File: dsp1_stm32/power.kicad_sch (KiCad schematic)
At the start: 41 parts, among them U10 TLV62568DBV, U9 TLV62568DBV

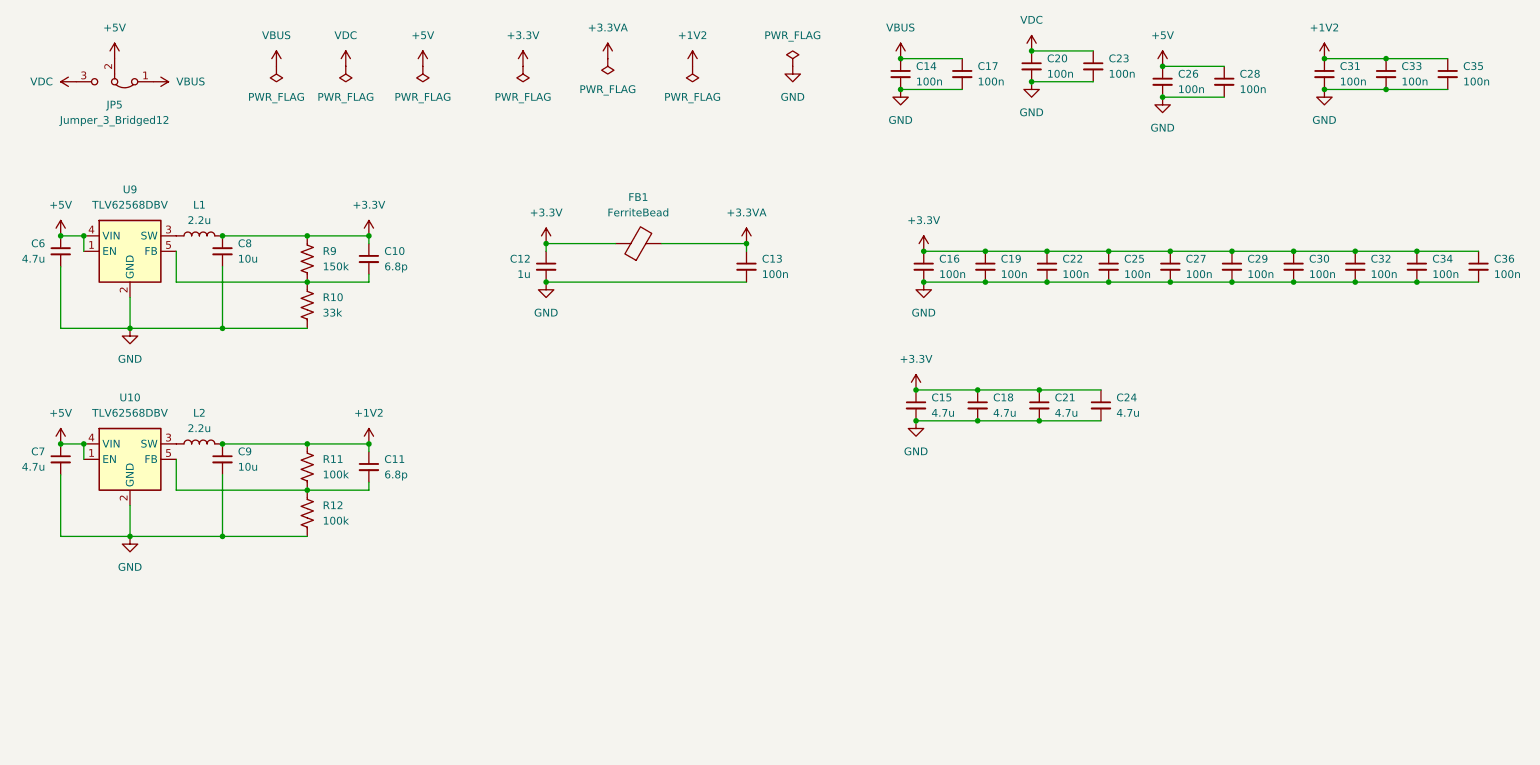
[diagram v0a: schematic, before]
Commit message: Circuit done
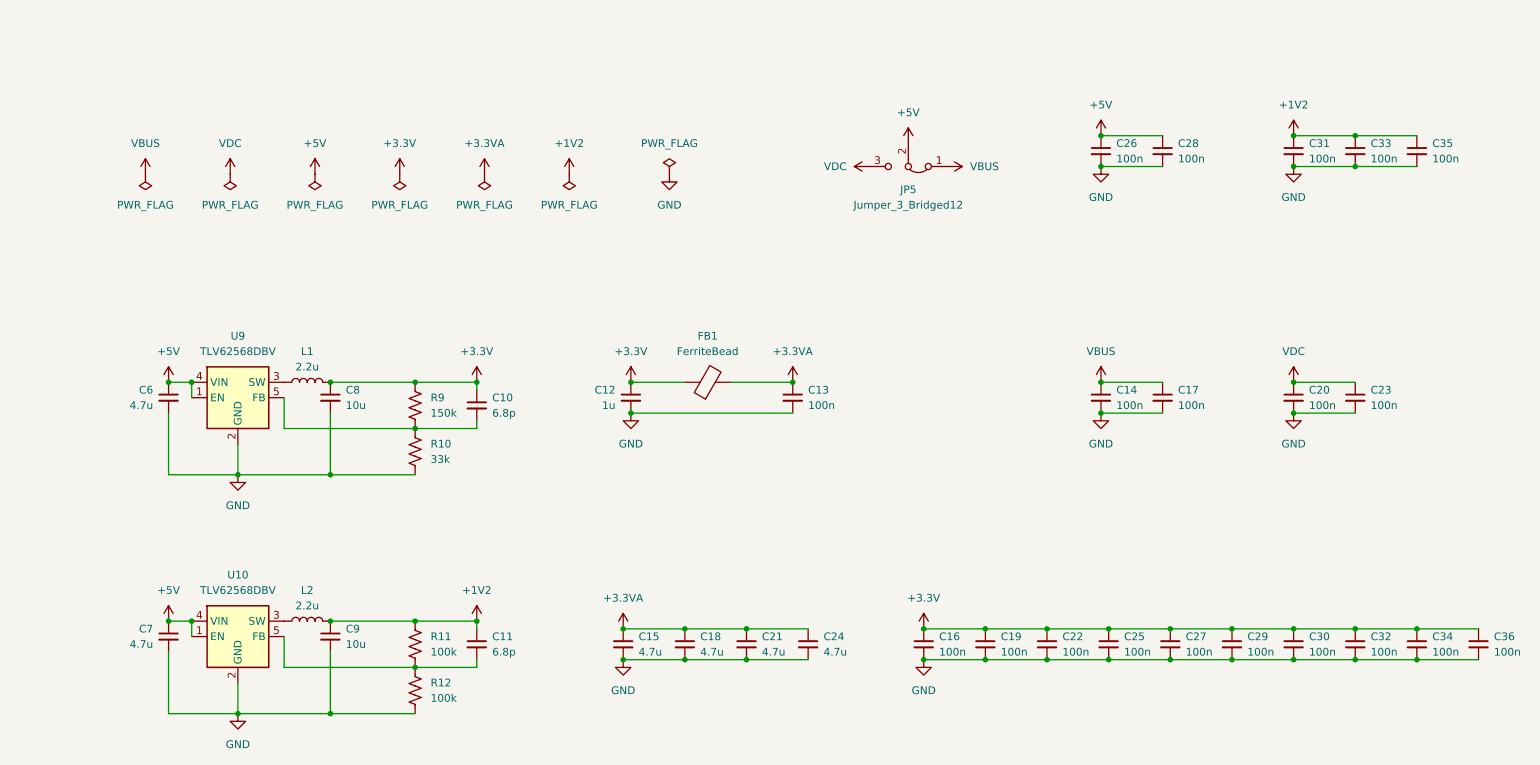
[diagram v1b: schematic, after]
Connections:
- net +3.3V: no longer C15.1, C18.1, C21.1, C24.1
- net +3.3VA: now also C15.1, C18.1, C21.1, C24.1
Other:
- moved on the sheet: C10, C11, C12, C13, C14, C15, C16, C17, C18, C19, C20, C21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
